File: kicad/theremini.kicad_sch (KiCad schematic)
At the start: 2 parts, among them U1 VL53L0CXV0DH/1, U2 VL53L0CXV0DH/1

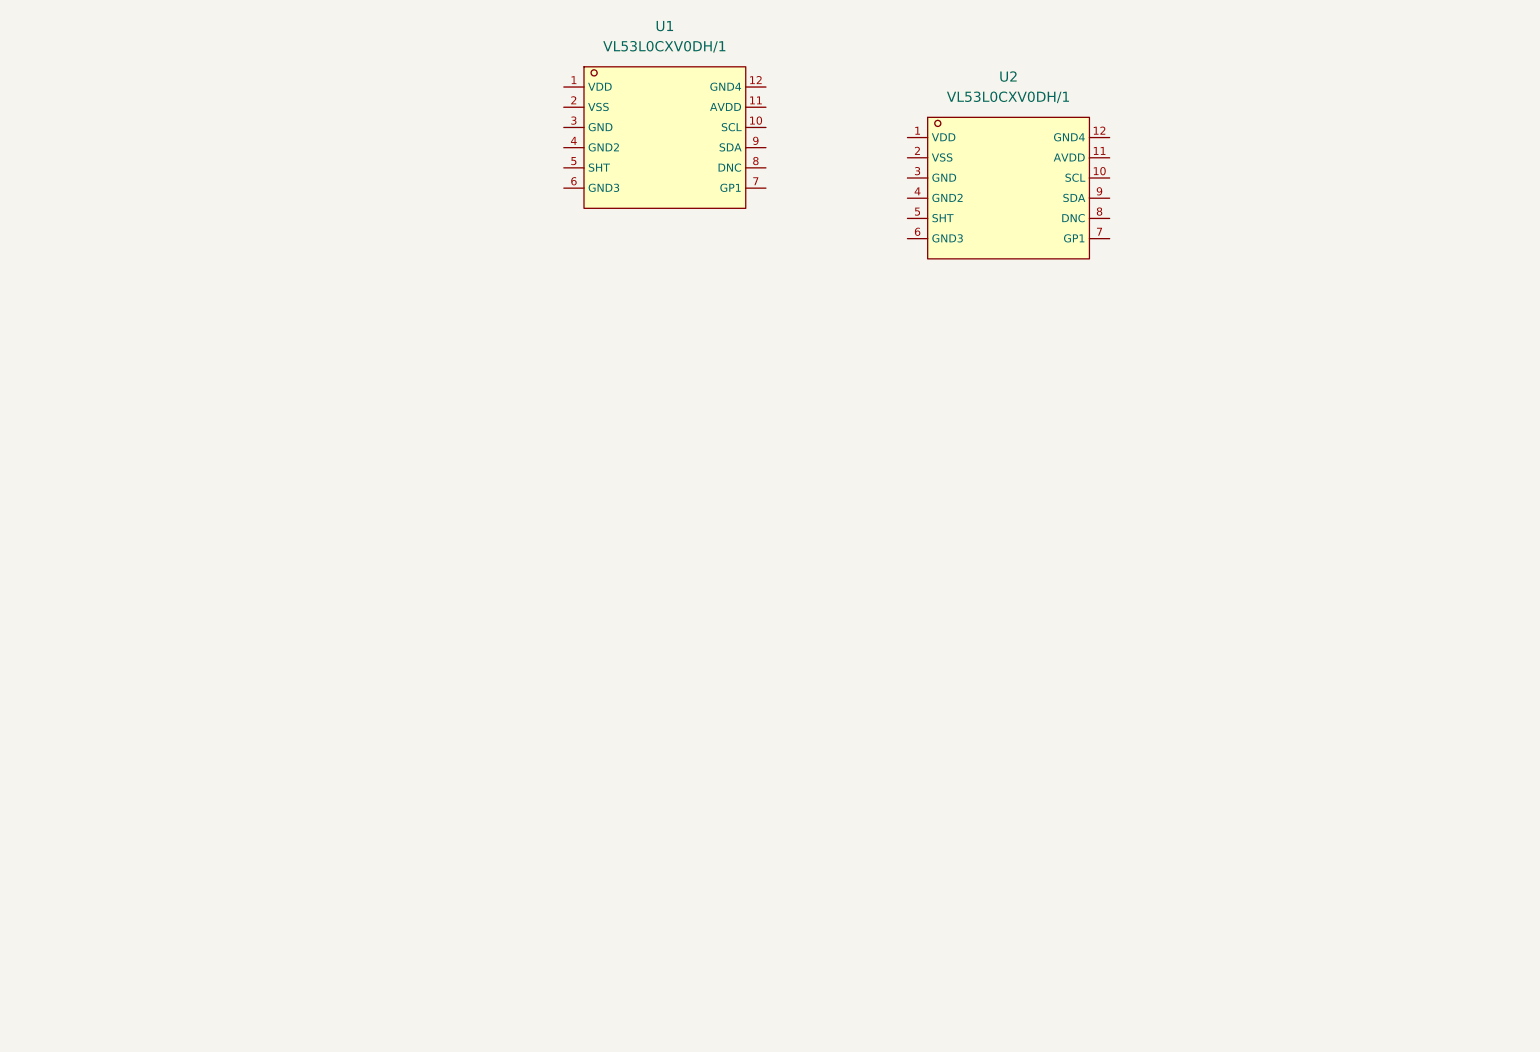
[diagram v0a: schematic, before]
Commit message: Add libraries
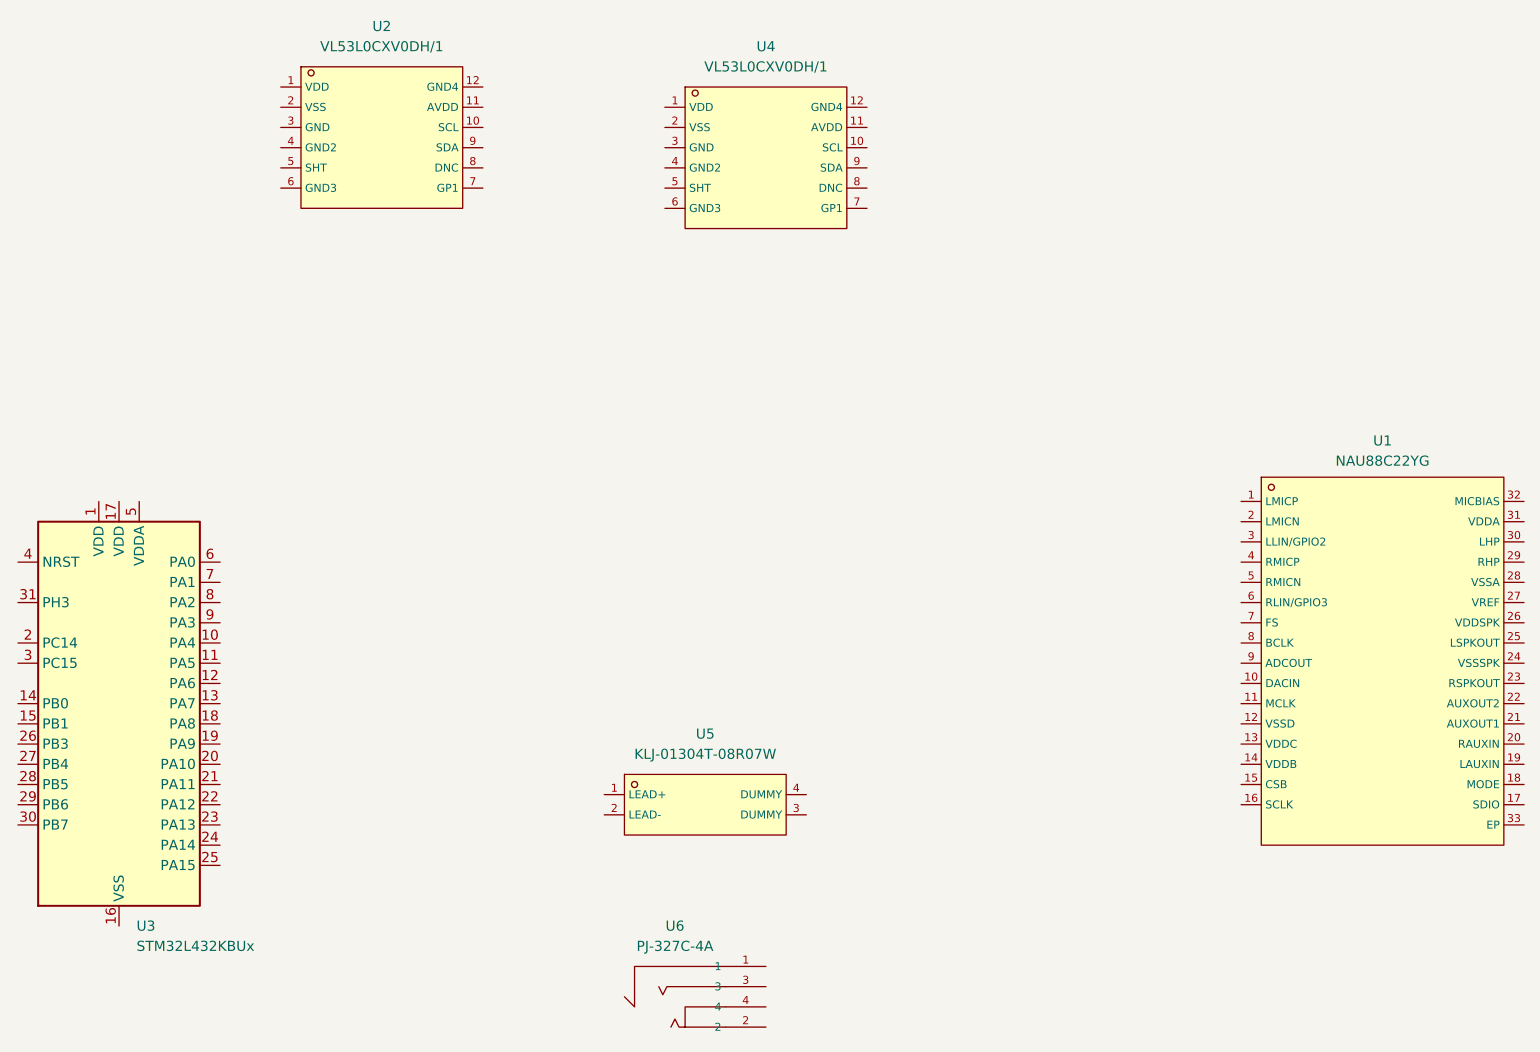
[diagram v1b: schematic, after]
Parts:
- removed U1: VL53L0CXV0DH/1, VL53L0CXV0DH1:OPTO-SMD_12P_VL53L0CXV0DH-1, symbol VL53L0CXV0DH/1:VL53L0CXV0DH/1
- added U1: NAU88C22YG, NAU88C22YG:QFN-32_L5.0-W5.0-P0.50-BL-EP3.4, symbol NAU88C22YG:NAU88C22YG
- added U3: STM32L432KBUx, Package_DFN_QFN:QFN-32-1EP_5x5mm_P0.5mm_EP3.45x3.45mm, symbol MCU_ST_STM32L4:STM32L432KBUx
- added U4: VL53L0CXV0DH/1, VL53L0CXV0DH1:OPTO-SMD_12P_VL53L0CXV0DH-1, symbol VL53L0CXV0DH/1:VL53L0CXV0DH/1
- added U5: KLJ-01304T-08R07W, KLJ-01304T-08R07W:BUZ-SMD_4P-L13.0-W13.0-P11.4-BL, symbol KLJ-01304T-08R07W:KLJ-01304T-08R07W
- added U6: PJ-327C-4A, PJ-327C-4A:AUDIO-SMD_PJ-327C-4A, symbol PJ-327C-4A:PJ-327C-4A
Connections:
- new net: U3.16 (VSS), U3.32 (VSS), U3.33 (VSS)
